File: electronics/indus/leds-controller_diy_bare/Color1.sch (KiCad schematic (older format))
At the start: 18 parts, among them U4 TPS92513HVDGQT

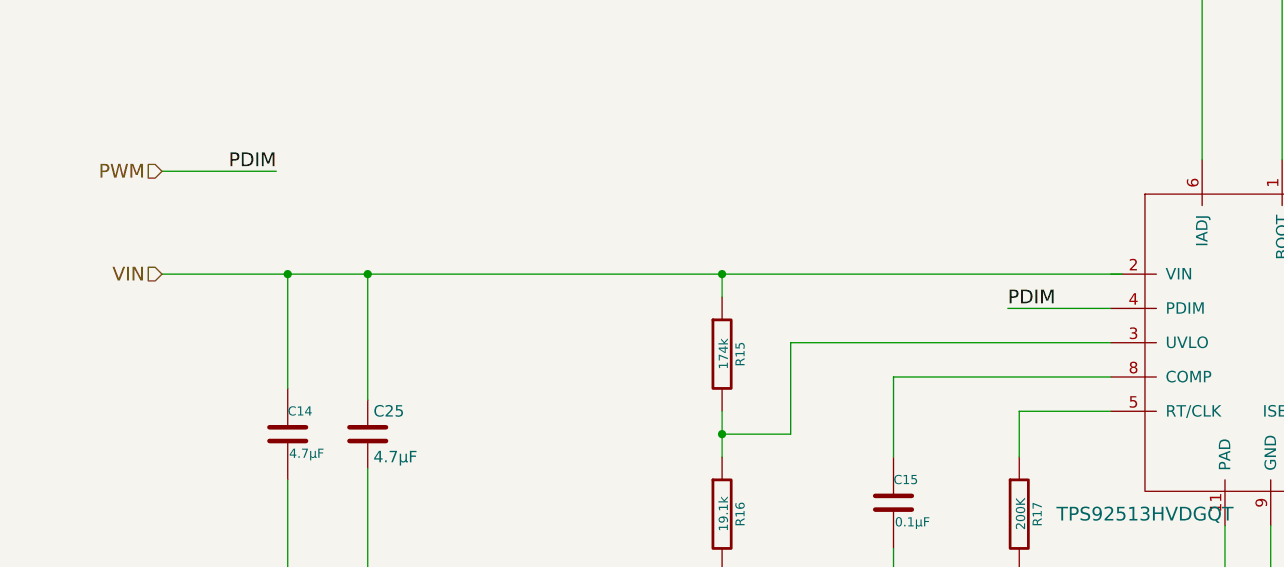
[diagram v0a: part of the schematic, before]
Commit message: fix some errors
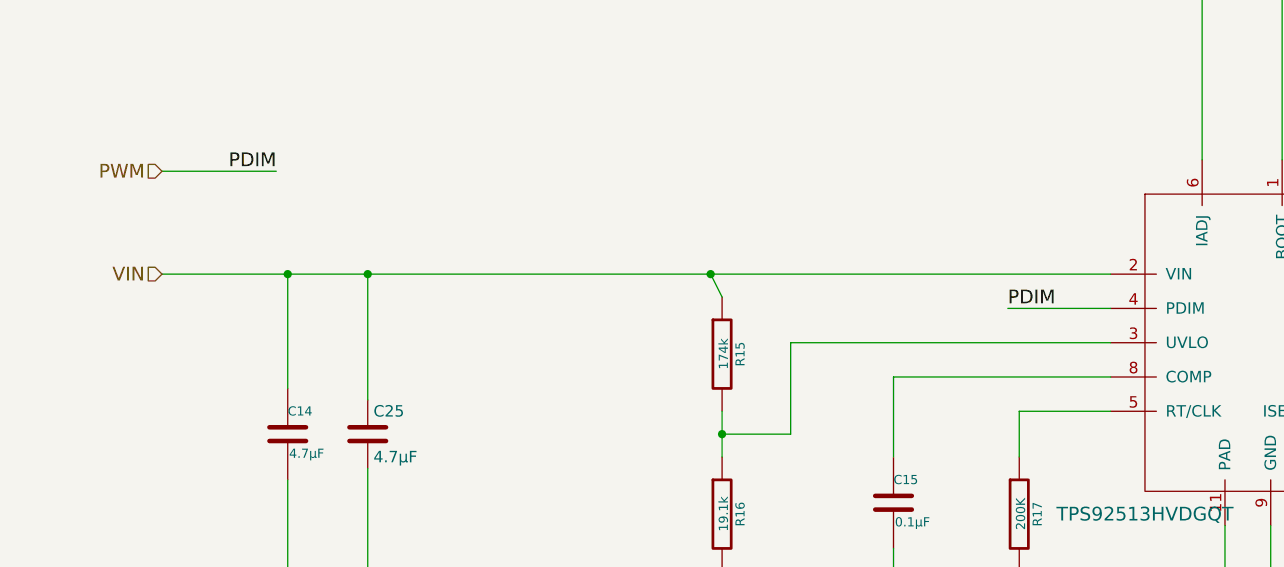
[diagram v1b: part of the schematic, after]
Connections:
- net VIN: now also U4.2 (VIN)
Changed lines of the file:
@@
 POT_OUT
 Wire Wire Line
-	1100 3450 5300 3450
+	1100 3450 5250 3450
 Wire Wire Line
 	1650 4900 10150 4900
@@
 	3550 4750 3550 4900
 Wire Wire Line
-	3550 3550 3550 3450
-Connection ~ 3550 3450
+	3550 3550 3500 3450
+Connection ~ 3500 3450
 Connection ~ 3550 4900
 Wire Wire Line
